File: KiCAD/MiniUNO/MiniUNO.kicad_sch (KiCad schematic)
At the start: 28 parts, among them IC1 AZ1117CR2-5.0TRG1, J1 USB_B_Micro, J2 Conn_01x11, J3 Conn_01x11, J4 Conn_01x07, Q1 FDN340P, Q2 PMV48XP, U1 ATmega32U4-A, Y1 830108288709

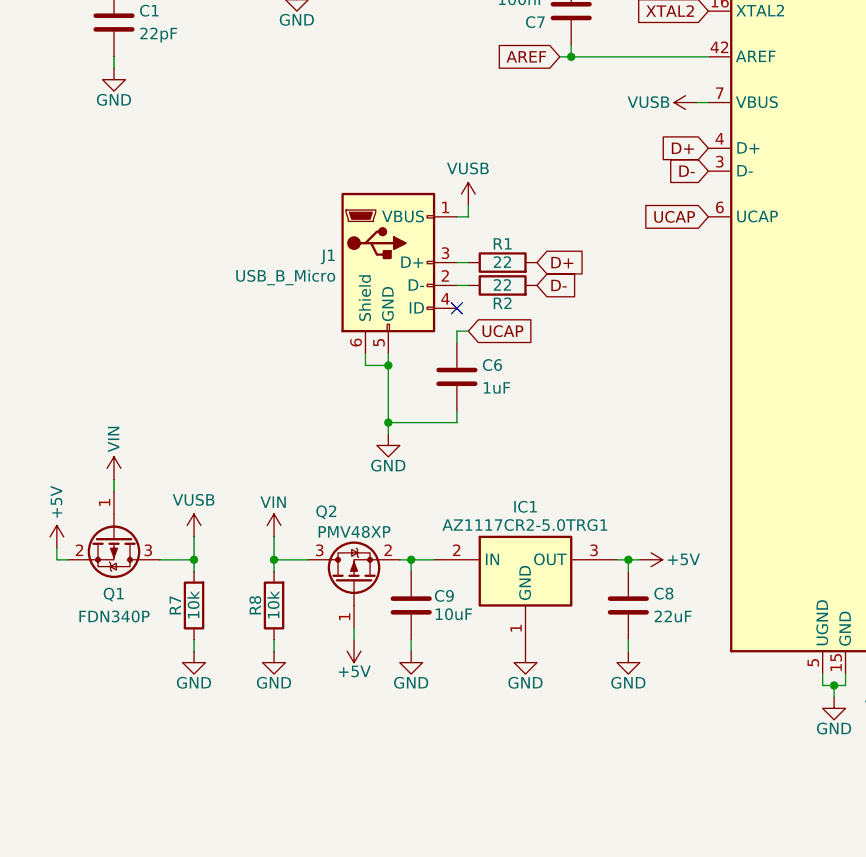
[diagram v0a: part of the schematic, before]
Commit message: Finalized design v1
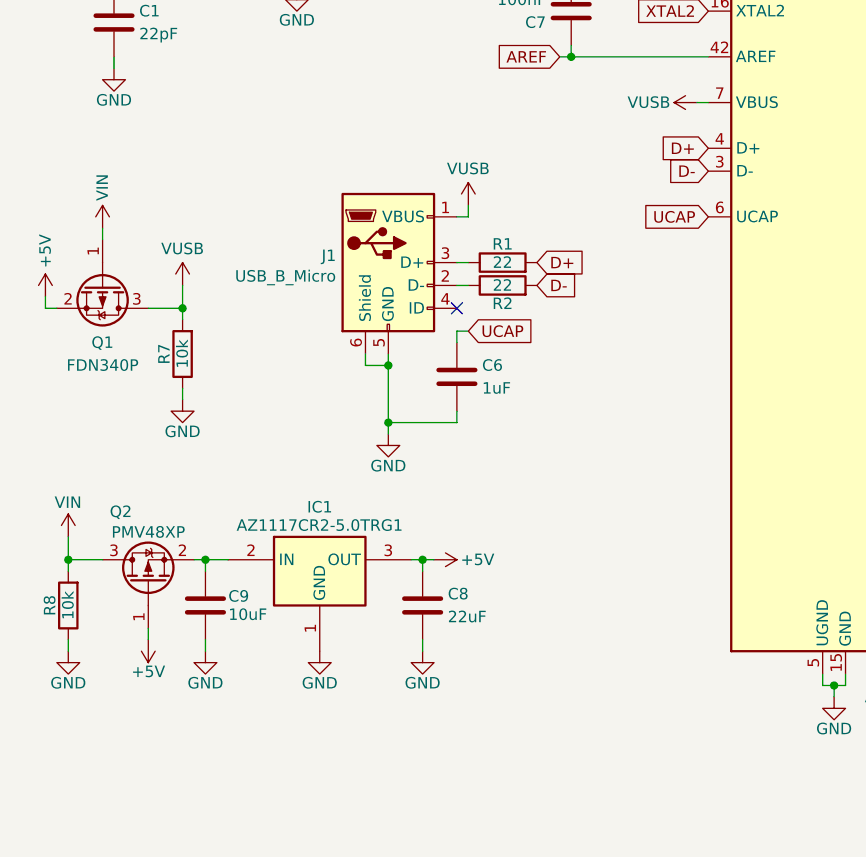
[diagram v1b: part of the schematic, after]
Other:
- moved on the sheet: C8, C9, IC1, Q1, Q2, R7, R8
